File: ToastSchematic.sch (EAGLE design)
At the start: 86 parts, among them Q1 DMN63D8LDW, Q2 DMN63D8LDW, Q3 DMN63D8LDW, Q4 DMN63D8LDW, T1 BPX81, T2 BPX81, T3 BPX81, T4 BPX81, T5 BPX81, T6 BPX81, U3 DRV8839_DSS_12, U4 DRV8839_DSS_12

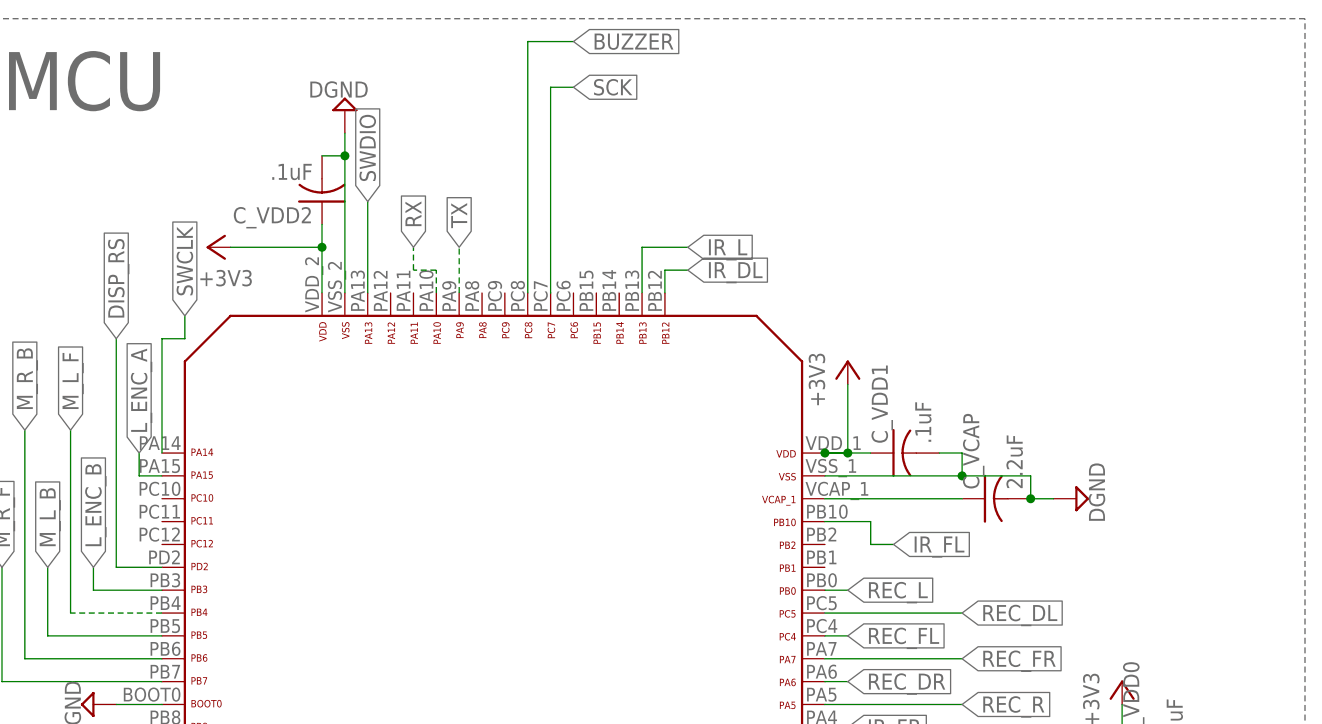
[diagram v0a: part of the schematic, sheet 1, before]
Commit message: finished wiring everything
still need to add toast and butter pics on the back and smash and label
stuff
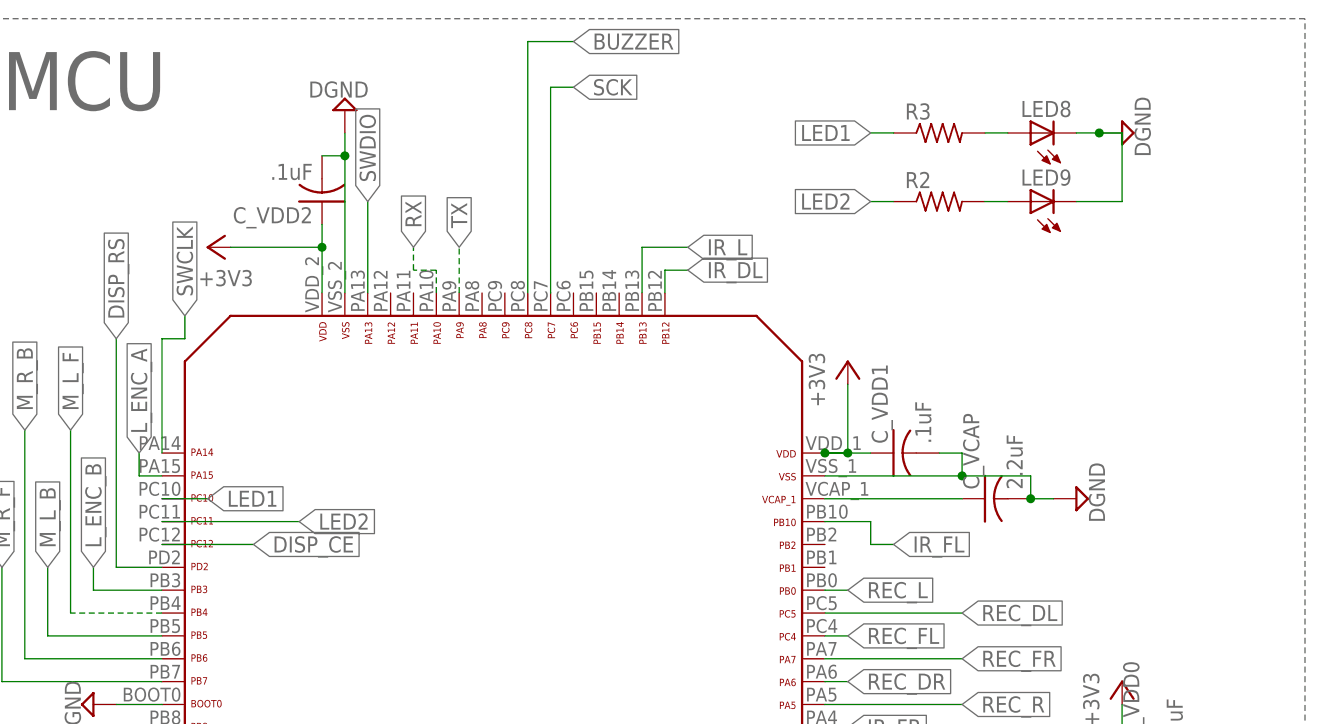
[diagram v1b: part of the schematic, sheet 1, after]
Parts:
- added LED8, LED9: (no value), led:LEDCHIPLED_0603
- added R2, R3: (no value), resistor:R-US_R0603
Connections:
- new net LED1: R3.1, U$1.PC10
- new net LED2: R2.1, U$1.PC11
- new net N$22: LED8.A, R3.2
- new net N$25: LED9.A, R2.2
- net DGND: now also LED8.C, LED9.C
- net DISP_CE: now also U$1.PC12
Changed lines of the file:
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@@
 <?xml version="1.0" encoding="utf-8"?>
 <!DOCTYPE eagle SYSTEM "eagle.dtd">
-<eagle version="8.3.1">
+<eagle version="8.4.1">
 <drawing>
 <settings>
@@
 <part name="SUPPLY46" library="SparkFun-PowerSymbols" deviceset="V_BATT" device=""/>
 <part name="SUPPLY47" library="supply2" library_urn="urn:adsk.eagle:library:372" deviceset="GND" device=""/>
+<part name="R2" library="resistor" library_urn="urn:adsk.eagle:library:348" deviceset="R-US_" device="R0603" package3d_urn="urn:adsk.eagle:package:26057/1"/>
+<part name="R3" library="resistor" library_urn="urn:adsk.eagle:library:348" deviceset="R-US_" device="R0603" package3d_urn="urn:adsk.eagle:package:26057/1"/>
+<part name="LED8" library="led" library_urn="urn:adsk.eagle:library:259" deviceset="LED" device="CHIPLED_0603" package3d_urn="urn:adsk.eagle:package:15822/1"/>
+<part name="LED9" library="led" library_urn="urn:adsk.eagle:library:259" deviceset="LED" device="CHIPLED_0603" package3d_urn="urn:adsk.eagle:package:15822/1"/>
+<part name="SUPPLY48" library="supply2" library_urn="urn:adsk.eagle:library:372" deviceset="DGND" device=""/>
 </parts>
 <sheets>
@@
 <instance part="SUPPLY46" gate="G$1" x="63.5" y="142.24"/>
 <instance part="SUPPLY47" gate="GND" x="88.9" y="129.54"/>
+<instance part="R2" gate="G$1" x="213.36" y="152.4"/>
+<instance part="R3" gate="G$1" x="213.36" y="160.02"/>
+<instance part="LED8" gate="G$1" x="223.52" y="160.02" rot="R90"/>
+<instance part="LED9" gate="G$1" x="223.52" y="152.4" rot="R90"/>
+<instance part="SUPPLY48" gate="G$1" x="233.68" y="160.02" rot="R90"/>
 </instances>
 <busses>
@@
 <pinref part="U$5" gate="G$1" pin="2"/>
 <wire x1="33.02" y1="137.16" x2="35.56" y2="137.16" width="0.1524" layer="91"/>
+</segment>
+<segment>
+<pinref part="LED8" gate="G$1" pin="C"/>
+<wire x1="228.6" y1="160.02" x2="231.14" y2="160.02" width="0.1524" layer="91"/>
+<pinref part="SUPPLY48" gate="G$1" pin="DGND"/>
+<pinref part="LED9" gate="G$1" pin="C"/>
+<wire x1="228.6" y1="152.4" x2="233.68" y2="152.4" width="0.1524" layer="91"/>
+<wire x1="233.68" y1="152.4" x2="233.68" y2="160.02" width="0.1524" layer="91"/>
+<wire x1="233.68" y1="160.02" x2="231.14" y2="160.02" width="0.1524" layer="91"/>
+<junction x="231.14" y="160.02"/>
 </segment>
 </net>
@@
 </segment>
 </net>
+<net name="DISP_CE" class="0">
+<segment>
+<pinref part="U$1" gate="G$1" pin="PC12"/>
+<wire x1="127" y1="114.3" x2="137.16" y2="114.3" width="0.1524" layer="91"/>
+<label x="137.16" y="114.3" size="1.778" layer="95" xref="yes"/>
+</segment>
+</net>
+<net name="N$22" class="0">
+<segment>
+<pinref part="R3" gate="G$1" pin="2"/>
+<pinref part="LED8" gate="G$1" pin="A"/>
+<wire x1="218.44" y1="160.02" x2="220.98" y2="160.02" width="0.1524" layer="91"/>
+</segment>
+</net>
+<net name="LED1" class="0">
+<segment>
+<pinref part="U$1" gate="G$1" pin="PC10"/>
+<wire x1="127" y1="119.38" x2="132.08" y2="119.38" width="0.1524" layer="91"/>
+<label x="132.08" y="119.38" size="1.778" layer="95" xref="yes"/>
+</segment>
+<segment>
+<pinref part="R3" gate="G$1" pin="1"/>
+<wire x1="208.28" y1="160.02" x2="205.74" y2="160.02" width="0.1524" layer="91"/>
+<label x="205.74" y="160.02" size="1.778" layer="95" rot="R180" xref="yes"/>
+</segment>
+</net>
+<net name="LED2" class="0">
+<segment>
+<pinref part="U$1" gate="G$1" pin="PC11"/>
+<wire x1="127" y1="116.84" x2="142.24" y2="116.84" width="0.1524" layer="91"/>
+<label x="142.24" y="116.84" size="1.778" layer="95" xref="yes"/>
+</segment>
+<segment>
+<pinref part="R2" gate="G$1" pin="1"/>
+<wire x1="208.28" y1="152.4" x2="205.74" y2="152.4" width="0.1524" layer="91"/>
+<label x="205.74" y="152.4" size="1.778" layer="95" rot="R180" xref="yes"/>
+</segment>
+</net>
+<net name="N$25" class="0">
+<segment>
+<pinref part="R2" gate="G$1" pin="2"/>
+<pinref part="LED9" gate="G$1" pin="A"/>
+<wire x1="218.44" y1="152.4" x2="220.98" y2="152.4" width="0.1524" layer="91"/>
+</segment>
+</net>
